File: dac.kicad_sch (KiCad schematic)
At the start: 18 parts, among them IC7 UDA1334BTS_N2,112

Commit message: finalize power and esp schemas
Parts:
- 4C1, 4C10, 4C2, 4C6, 4C8: footprint (none) -> Capacitor_SMD:C_0402_1005Metric
- 4C3, 4C4, 4C5, 4C7, 4C9: footprint (none) -> Capacitor_Tantalum_SMD:CP_EIA-3528-21_Kemet-B
- 4R1, 4R2, 4R3, 4R4, 4R6, 4R7, 4R8: footprint (none) -> Resistor_SMD:R_0402_1005Metric
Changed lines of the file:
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@@
 			)
 		)
-		(property "Footprint" ""
+		(property "Footprint" "Capacitor_Tantalum_SMD:CP_EIA-3528-21_Kemet-B"
 			(at 99.06 41.6052 0)
 			(hide yes)
@@
 			)
 		)
-		(property "Footprint" ""
+		(property "Footprint" "Capacitor_SMD:C_0402_1005Metric"
 			(at 99.06 56.8452 0)
 			(hide yes)
@@
 			)
 		)
-		(property "Footprint" ""
+		(property "Footprint" "Capacitor_Tantalum_SMD:CP_EIA-3528-21_Kemet-B"
 			(at 148.59 41.6052 0)
 			(hide yes)
@@
 			)
 		)
-		(property "Footprint" ""
+		(property "Footprint" "Capacitor_SMD:C_0402_1005Metric"
 			(at 176.2252 146.05 0)
 			(hide yes)
@@
 			)
 		)
-		(property "Footprint" ""
+		(property "Footprint" "Resistor_SMD:R_0402_1005Metric"
 			(at 199.39 84.328 90)
 			(hide yes)
@@
 			)
 		)
-		(property "Footprint" ""
+		(property "Footprint" "Capacitor_Tantalum_SMD:CP_EIA-3528-21_Kemet-B"
 			(at 185.42 81.5848 0)
 			(hide yes)
@@
 			)
 		)
-		(property "Footprint" ""
+		(property "Footprint" "Resistor_SMD:R_0402_1005Metric"
 			(at 187.452 91.44 90)
 			(hide yes)
@@
 			)
 		)
-		(property "Footprint" ""
+		(property "Footprint" "Resistor_SMD:R_0402_1005Metric"
 			(at 199.39 110.998 90)
 			(hide yes)
@@
 			)
 		)
-		(property "Footprint" ""
+		(property "Footprint" "Resistor_SMD:R_0402_1005Metric"
 			(at 110.998 116.84 90)
 			(hide yes)
@@
 			)
 		)
-		(property "Footprint" ""
+		(property "Footprint" "Resistor_SMD:R_0402_1005Metric"
 			(at 187.452 118.11 90)
 			(hide yes)
@@
 			)
 		)
-		(property "Footprint" ""
+		(property "Footprint" "Capacitor_SMD:C_0402_1005Metric"
 			(at 210.5152 95.25 0)
 			(hide yes)
@@
 			)
 		)
-		(property "Footprint" ""
+		(property "Footprint" "Capacitor_Tantalum_SMD:CP_EIA-3528-21_Kemet-B"
 			(at 195.2752 146.05 0)
 			(hide yes)
@@
 			)
 		)
-		(property "Footprint" ""
+		(property "Footprint" "Capacitor_Tantalum_SMD:CP_EIA-3528-21_Kemet-B"
 			(at 185.42 108.2548 0)
 			(hide yes)
@@
 			)
 		)
-		(property "Footprint" ""
+		(property "Footprint" "Resistor_SMD:R_0402_1005Metric"
 			(at 113.792 30.48 90)
 			(hide yes)
@@
 			)
 		)
-		(property "Footprint" ""
+		(property "Footprint" "Capacitor_SMD:C_0402_1005Metric"
 			(at 148.59 56.8452 0)
 			(hide yes)
@@
 			)
 		)
-		(property "Footprint" ""
+		(property "Footprint" "Resistor_SMD:R_0402_1005Metric"
 			(at 163.322 30.48 90)
 			(hide yes)
@@
 			)
 		)
-		(property "Footprint" ""
+		(property "Footprint" "Capacitor_SMD:C_0402_1005Metric"
 			(at 210.5152 121.92 0)
 			(hide yes)

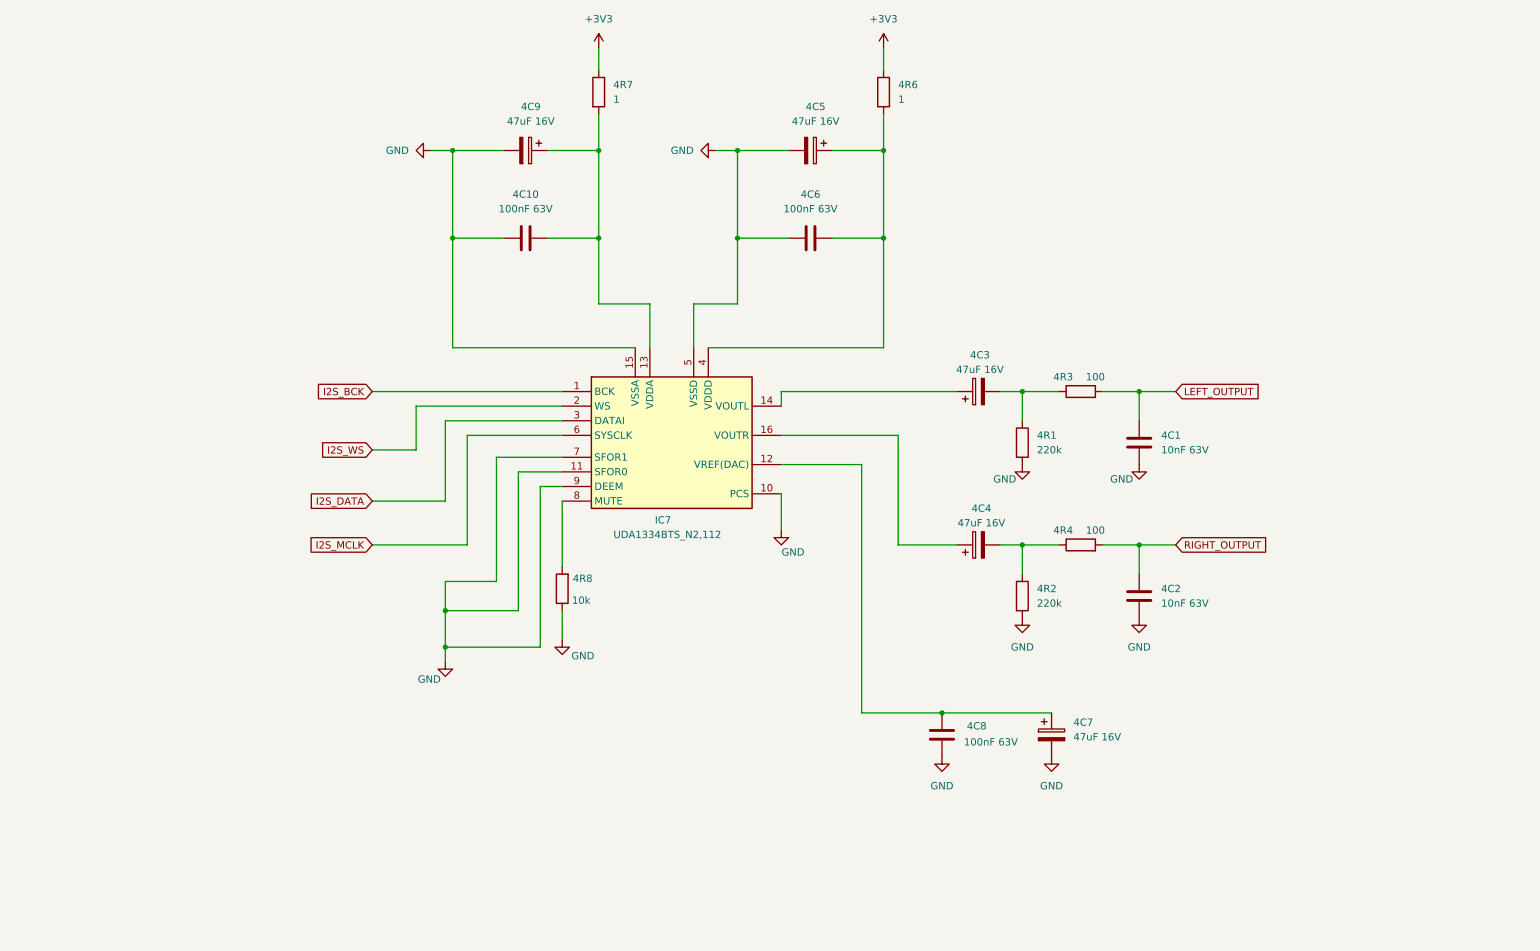
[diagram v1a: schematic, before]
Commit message: finalized schema
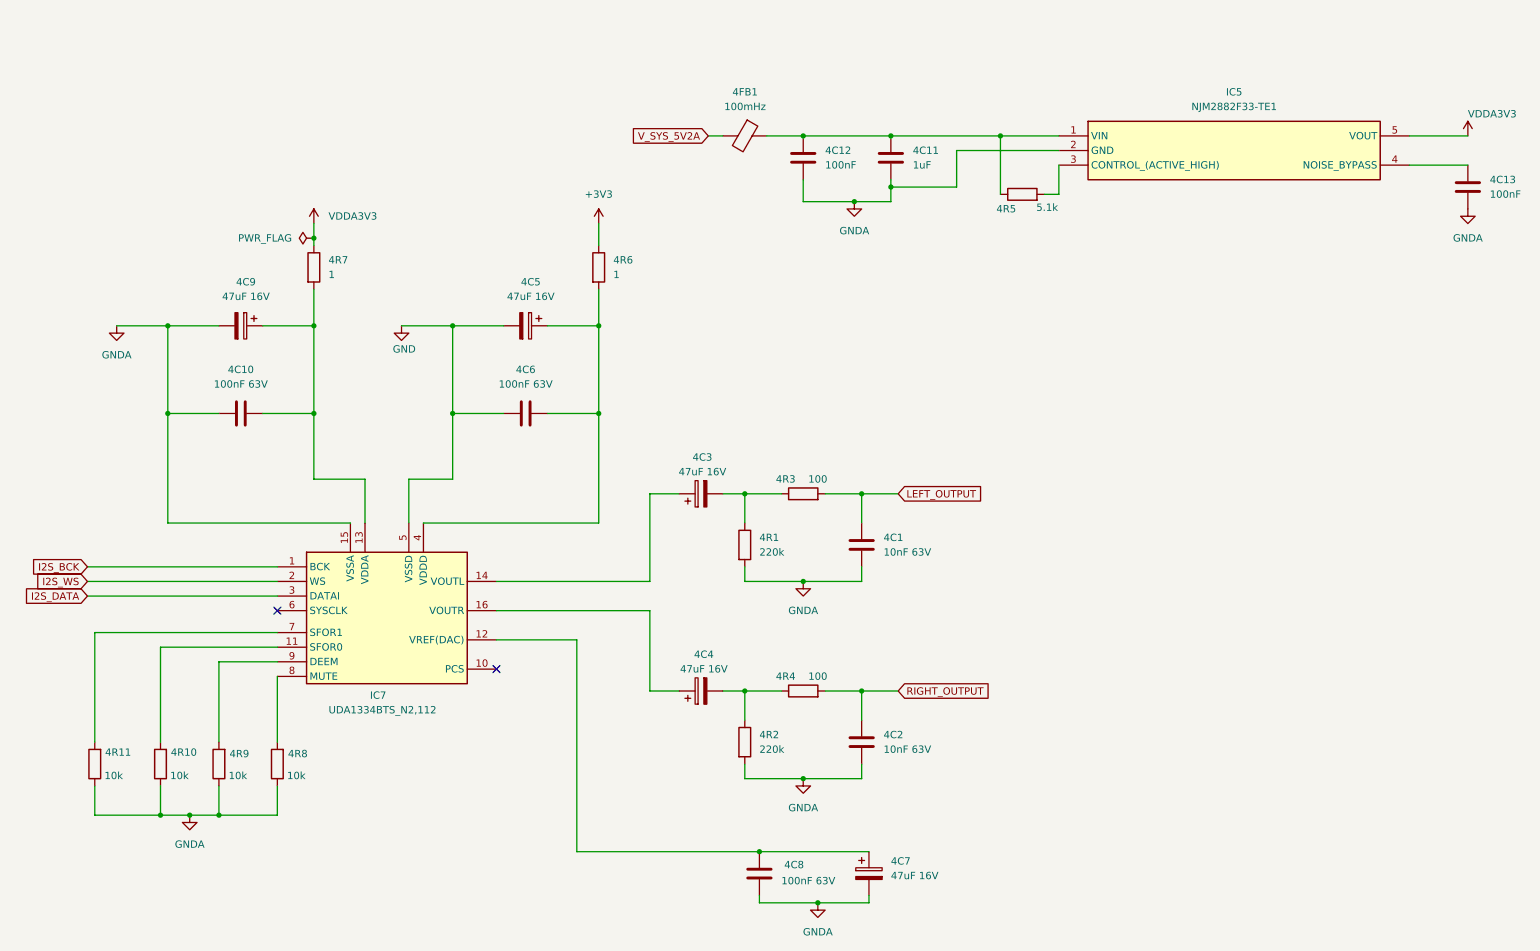
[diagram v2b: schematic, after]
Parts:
- added 4C11: 1uF, Capacitor_SMD:C_0402_1005Metric, symbol Device:C
- added 4C12, 4C13: 100nF, Capacitor_SMD:C_0402_1005Metric, symbol Device:C
- added 4FB1: 100mHz, Inductor_SMD:L_0402_1005Metric, symbol Device:FerriteBead
- added 4R10, 4R11, 4R9: 10k, Resistor_SMD:R_0402_1005Metric, symbol Device:R
- added 4R5: 5.1k, Resistor_SMD:R_0402_1005Metric, symbol Device:R
- added IC5: NJM2882F33-TE1, ipradio:SOT95P280X130-5N, symbol ipradio:NJM2882F33-TE1
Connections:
- net +3V3: no longer 4R7.1
- net GND: no longer 4C1.2, 4C10.2, 4C2.2, 4C7.2, 4C8.2, 4C9.2, 4R1.2, 4R2.2, 4R8.1, IC7.10 (PCS), IC7.11 (SFOR0), IC7.15 (VSSA), IC7.7 (SFOR1), IC7.9 (DEEM)
- net I2S_MCLK: no longer names the net of IC7.6 (SYSCLK)
- new net: 4R9.2, IC7.9 (DEEM)
- new net: 4C13.1, IC5.4 (NOISE_BYPASS)
- new net: 4C11.1, 4C12.1, 4FB1.1, 4R5.1, IC5.1 (VIN)
- new net: 4R10.2, IC7.11 (SFOR0)
- new net: 4R11.2, IC7.7 (SFOR1)
- new net: 4R5.2, IC5.3 (CONTROL_(ACTIVE_HIGH))
- new net GNDA: 4C1.2, 4C10.2, 4C11.2, 4C12.2, 4C13.2, 4C2.2, 4C7.2, 4C8.2, 4C9.2, 4R1.2, 4R10.1, 4R11.1, 4R2.2, 4R8.1, 4R9.1, IC5.2 (GND), IC7.15 (VSSA)
- new net VDDA3V3: 4R7.1, IC5.5 (VOUT)
- new net V_SYS_5V2A: 4FB1.2
- no-connect marks 0 -> 2
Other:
- moved on the sheet: 4C1, 4C10, 4C2, 4C3, 4C4, 4C5, 4C6, 4C7, 4C8, 4C9, 4R1, 4R2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
